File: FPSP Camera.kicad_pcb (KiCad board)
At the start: 4 copper layers, 85.7 x 35 mm, 80 parts, among them J2 Conn_01x02_Pin, J3 USB_B_Micro, J4 SM03B-SRSS-TB, J5 Conn_01x24_Socket, J6 Conn_02x06_Odd_Even, SW1 SW_Push, SW2 SW_Push, U1 RP2350_60QFN, U2 W25Q128JVS, U3 ASM330LHHXTR, U5 TLV74328_SOT23-5, U6 TLV74315_SOT23-5, U7 SiT2001B, U8 NCP1117-3.3_SOT223

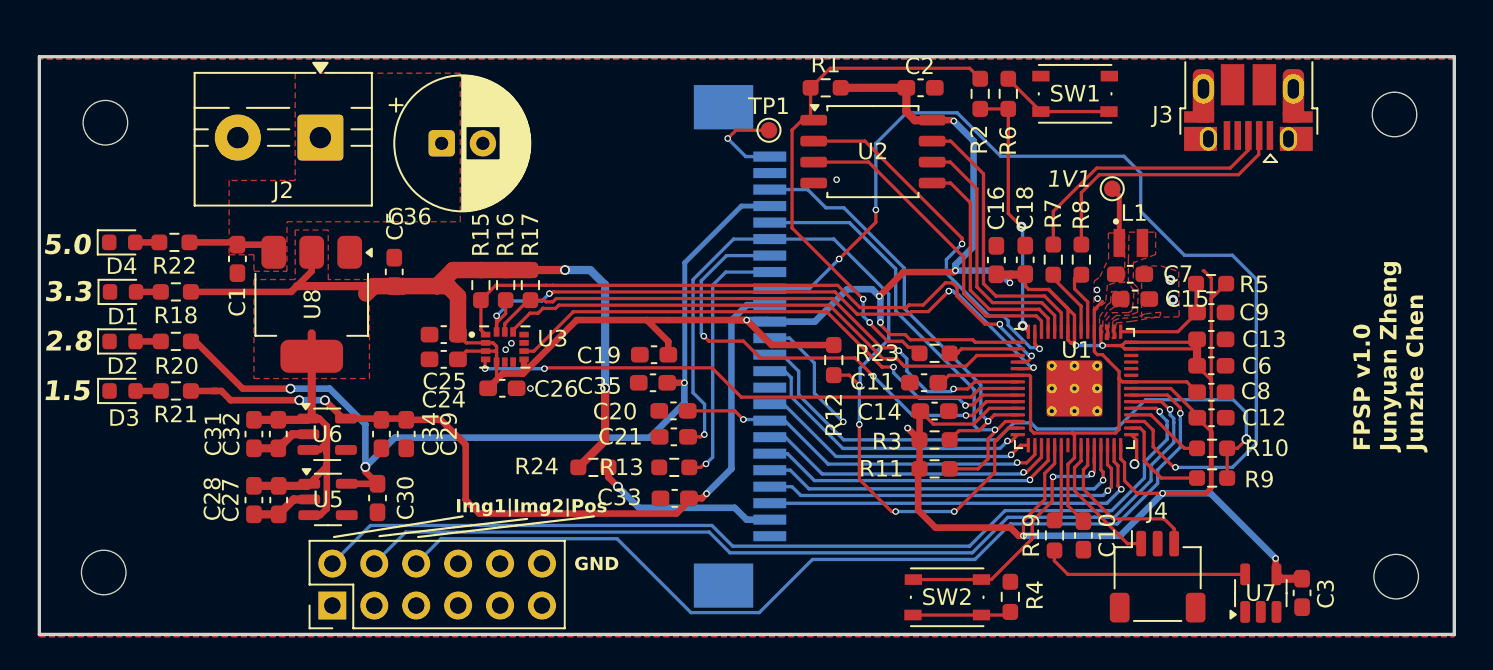
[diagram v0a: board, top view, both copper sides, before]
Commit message: Cleanup
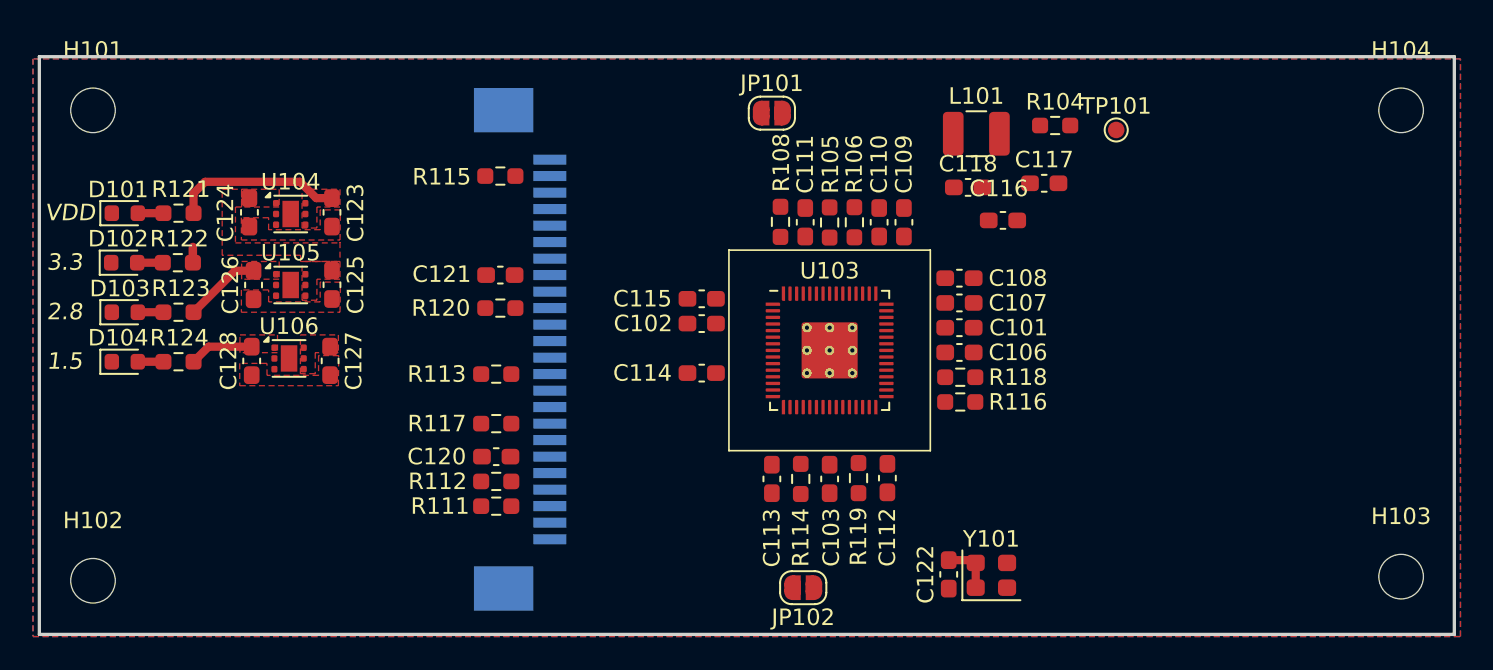
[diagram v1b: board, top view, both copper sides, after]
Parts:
- removed C1, C19, C25, C27, C28, C30, C31, C32, C33, C34, C35, C5: 10u, Capacitor_SMD:C_0603_1608Metric_Pad1.08x0.95mm_HandSolder
- removed C10, C6, C7, C9: 4.7u, Capacitor_SMD:C_0603_1608Metric_Pad1.08x0.95mm_HandSolder
- removed C11, C12, C13, C14, C15, C16, C18, C2, C24, C26, C8: 100n, Capacitor_SMD:C_0603_1608Metric_Pad1.08x0.95mm_HandSolder
- removed C20: 22pF, Capacitor_SMD:C_0603_1608Metric_Pad1.08x0.95mm_HandSolder
- removed C21: 0.1u, Capacitor_SMD:C_0603_1608Metric_Pad1.08x0.95mm_HandSolder
- removed C29: 1u, Capacitor_SMD:C_0603_1608Metric_Pad1.08x0.95mm_HandSolder
- removed C3: 100u, Capacitor_SMD:C_0603_1608Metric_Pad1.08x0.95mm_HandSolder
- removed C36: 10u, Capacitor_THT:CP_Radial_D8.0mm_P2.50mm
- removed D1, D2, D3, D4: LED, Diode_SMD:D_0603_1608Metric
- removed H1, H2, H3, H4: MountingHole, MountingHole:MountingHole_2.7mm_M2.5
- removed J2: Conn_01x02_Pin, TerminalBlock:TerminalBlock_MaiXu_MX126-5.0-02P_1x02_P5.00mm
- removed J3: USB_B_Micro, RP2350_60QFN_minimal:USB_Micro-B_Amphenol_10103594-0001LF_Horizontal_modified
- removed J4: SM03B-SRSS-TB, Connector_JST:JST_SH_SM03B-SRSS-TB_1x03-1MP_P1.00mm_Horizontal
- removed J5: Conn_01x24_Socket, Connector_FFC-FPC:TE_2-84952-4_1x24-1MP_P1.0mm_Horizontal
- removed J6: Conn_02x06_Odd_Even, Connector_PinHeader_2.54mm:PinHeader_2x06_P2.54mm_Vertical
- removed L1: 3.3u, RP2350_60QFN_minimal:L_pol_2016
- removed R1, R19, R23: DNF, Resistor_SMD:R_0603_1608Metric_Pad0.98x0.95mm_HandSolder
- removed R10, R24, R9: 0R, Resistor_SMD:R_0603_1608Metric_Pad0.98x0.95mm_HandSolder
- removed R11, R12, R13, R15, R16, R17, R18, R20, R21, R22, R3: 10k, Resistor_SMD:R_0603_1608Metric_Pad0.98x0.95mm_HandSolder
- removed R2: 0, Resistor_SMD:R_0603_1608Metric_Pad0.98x0.95mm_HandSolder
- removed R4, R6: 1k, Resistor_SMD:R_0603_1608Metric_Pad0.98x0.95mm_HandSolder
- removed R5: 33, Resistor_SMD:R_0603_1608Metric_Pad0.98x0.95mm_HandSolder
- removed R7, R8: 27, Resistor_SMD:R_0603_1608Metric_Pad0.98x0.95mm_HandSolder
- removed SW1, SW2: SW_Push, Button_Switch_SMD:SW_Push_1P1T_NO_Vertical_Wuerth_434133025816
- removed TP1, TP2: TestPoint, TestPoint:TestPoint_Pad_D1.0mm
- removed U1: RP2350_60QFN, RP2350_60QFN_minimal:RP2350-QFN-60-1EP_7x7_P0.4mm_EP3.4x3.4mm_ThermalVias
- removed U2: W25Q128JVS, Package_SO:SOIC-8_5.3x5.3mm_P1.27mm
- removed U3: ASM330LHHXTR, ASM330LHHXTR:XDCR_ASM330LHHXTR
- removed U5: TLV74328_SOT23-5, Package_TO_SOT_SMD:SOT-23-5
- removed U6: TLV74315_SOT23-5, Package_TO_SOT_SMD:SOT-23-5
- removed U7: SiT2001B, Package_TO_SOT_SMD:SOT-23-5
- removed U8: NCP1117-3.3_SOT223, Package_TO_SOT_SMD:SOT-223-3_TabPin2
- added C101: 100n, Capacitor_SMD:C_0603_1608Metric_Pad1.08x0.95mm_HandSolder, F.Cu at (74.8, 28.9)
- added C102: 4.7u, Capacitor_SMD:C_0603_1608Metric_Pad1.08x0.95mm_HandSolder, F.Cu at (59.1, 28.7)
- added C103: 100n, Capacitor_SMD:C_0603_1608Metric_Pad1.08x0.95mm_HandSolder, F.Cu at (66.9, 38.1)
- added C106: 100n, Capacitor_SMD:C_0603_1608Metric_Pad1.08x0.95mm_HandSolder, F.Cu at (74.8, 30.4)
- added C107: 100n, Capacitor_SMD:C_0603_1608Metric_Pad1.08x0.95mm_HandSolder, F.Cu at (74.8, 27.4)
- added C108: 100n, Capacitor_SMD:C_0603_1608Metric_Pad1.08x0.95mm_HandSolder, F.Cu at (74.8, 25.9)
- added C109: 100n, Capacitor_SMD:C_0603_1608Metric_Pad1.08x0.95mm_HandSolder, F.Cu at (71.4, 22.6)
- added C110: 100n, Capacitor_SMD:C_0603_1608Metric_Pad1.08x0.95mm_HandSolder, F.Cu at (69.9, 22.6)
- added C111: 100n, Capacitor_SMD:C_0603_1608Metric_Pad1.08x0.95mm_HandSolder, F.Cu at (65.4, 22.6)
- added C112: 100n, Capacitor_SMD:C_0603_1608Metric_Pad1.08x0.95mm_HandSolder, F.Cu at (70.4, 38.0)
- added C113: 100n, Capacitor_SMD:C_0603_1608Metric_Pad1.08x0.95mm_HandSolder, F.Cu at (63.4, 38.1)
- added C114: 100n, Capacitor_SMD:C_0603_1608Metric_Pad1.08x0.95mm_HandSolder, F.Cu at (59.1, 31.7)
- added C115: 100n, Capacitor_SMD:C_0603_1608Metric_Pad1.08x0.95mm_HandSolder, F.Cu at (59.1, 27.2)
- added C116: 4.7u, Capacitor_SMD:C_0603_1608Metric_Pad1.08x0.95mm_HandSolder, F.Cu at (77.4, 22.4)
- added C117: 4.7u, Capacitor_SMD:C_0603_1608Metric_Pad1.08x0.95mm_HandSolder, F.Cu at (79.9, 20.2)
- added C118: 4.7u, Capacitor_SMD:C_0603_1608Metric_Pad1.08x0.95mm_HandSolder, F.Cu at (75.3, 20.4)
- added C120: 0.1u, Capacitor_SMD:C_0603_1608Metric_Pad1.08x0.95mm_HandSolder, F.Cu at (46.7, 36.8)
- added C121: 22pF, Capacitor_SMD:C_0603_1608Metric_Pad1.08x0.95mm_HandSolder, F.Cu at (47.0, 25.8)
- added C122: 100n, Capacitor_SMD:C_0603_1608Metric_Pad1.08x0.95mm_HandSolder, F.Cu at (74.1, 43.9)
- added C123: 1u, Capacitor_SMD:C_0603_1608Metric_Pad1.08x0.95mm_HandSolder, F.Cu at (36.8, 21.9)
- added C124: 1u, Capacitor_SMD:C_0603_1608Metric_Pad1.08x0.95mm_HandSolder, F.Cu at (31.8, 21.9)
- added C125: 1u, Capacitor_SMD:C_0603_1608Metric_Pad1.08x0.95mm_HandSolder, F.Cu at (36.8, 26.3)
- added C126: 1u, Capacitor_SMD:C_0603_1608Metric_Pad1.08x0.95mm_HandSolder, F.Cu at (32.0, 26.4)
- added C127: 1u, Capacitor_SMD:C_0603_1608Metric_Pad1.08x0.95mm_HandSolder, F.Cu at (36.6, 30.9)
- added C128: 1u, Capacitor_SMD:C_0603_1608Metric_Pad1.08x0.95mm_HandSolder, F.Cu at (31.9, 30.9)
- added D101: LED, Diode_SMD:D_0603_1608Metric, F.Cu at (24.2, 22.0)
- added D102: LED, Diode_SMD:D_0603_1608Metric, F.Cu at (24.2, 25.0)
- added D103: LED, Diode_SMD:D_0603_1608Metric, F.Cu at (24.2, 28.0)
- added D104: LED, Diode_SMD:D_0603_1608Metric, F.Cu at (24.2, 31.0)
- added H101: MountingHole, MountingHole:MountingHole_2.7mm_M2.5, F.Cu at (22.3, 15.8)
- added H102: MountingHole, MountingHole:MountingHole_2.7mm_M2.5, F.Cu at (22.3, 44.3)
- added H103: MountingHole, MountingHole:MountingHole_2.7mm_M2.5, F.Cu at (101.5, 44.0)
- added H104: MountingHole, MountingHole:MountingHole_2.7mm_M2.5, F.Cu at (101.5, 15.8)
- added J101: Conn_01x24_Socket, Connector_FFC-FPC:TE_2-84952-4_1x24-1MP_P1.0mm_Horizontal, B.Cu at (48.1, 30.2)
- added JP101: SolderJumper_2_Open, Jumper:SolderJumper-2_P1.3mm_Open_RoundedPad1.0x1.5mm, F.Cu at (63.4, 15.9)
- added JP102: SolderJumper_2_Open, Jumper:SolderJumper-2_P1.3mm_Open_RoundedPad1.0x1.5mm, F.Cu at (65.3, 44.7)
- added L101: 3.3u, Inductor_SMD:L_1210_3225Metric, F.Cu at (75.8, 17.2)
- added R104: 33, Resistor_SMD:R_0603_1608Metric_Pad0.98x0.95mm_HandSolder, F.Cu at (80.6, 16.7)
- added R105: 27, Resistor_SMD:R_0603_1608Metric_Pad0.98x0.95mm_HandSolder, F.Cu at (66.9, 22.6)
- added R106: 27, Resistor_SMD:R_0603_1608Metric_Pad0.98x0.95mm_HandSolder, F.Cu at (68.4, 22.6)
- added R108: 1k, Resistor_SMD:R_0603_1608Metric_Pad0.98x0.95mm_HandSolder, F.Cu at (63.9, 22.5)
- added R111: 10k, Resistor_SMD:R_0603_1608Metric_Pad0.98x0.95mm_HandSolder, F.Cu at (46.7, 39.8)
- added R112: 10k, Resistor_SMD:R_0603_1608Metric_Pad0.98x0.95mm_HandSolder, F.Cu at (46.7, 38.2)
- added R113: 10k, Resistor_SMD:R_0603_1608Metric_Pad0.98x0.95mm_HandSolder, F.Cu at (46.7, 31.8)
- added R114: DNF, Resistor_SMD:R_0603_1608Metric_Pad0.98x0.95mm_HandSolder, F.Cu at (65.2, 38.1)
- added R115: 0R, Resistor_SMD:R_0603_1608Metric_Pad0.98x0.95mm_HandSolder, F.Cu at (47.0, 19.8)
- added R116: 0R, Resistor_SMD:R_0603_1608Metric_Pad0.98x0.95mm_HandSolder, F.Cu at (74.8, 33.4)
- added R117: 10k, Resistor_SMD:R_0603_1608Metric_Pad0.98x0.95mm_HandSolder, F.Cu at (46.7, 34.8)
- added R118: 0R, Resistor_SMD:R_0603_1608Metric_Pad0.98x0.95mm_HandSolder, F.Cu at (74.8, 31.9)
- added R119: 1k, Resistor_SMD:R_0603_1608Metric_Pad0.98x0.95mm_HandSolder, F.Cu at (68.7, 38.0)
- added R120: 0R, Resistor_SMD:R_0603_1608Metric_Pad0.98x0.95mm_HandSolder, F.Cu at (47.0, 27.8)
- added R121: 10k, Resistor_SMD:R_0603_1608Metric_Pad0.98x0.95mm_HandSolder, F.Cu at (27.4, 22.0)
- added R122: 10k, Resistor_SMD:R_0603_1608Metric_Pad0.98x0.95mm_HandSolder, F.Cu at (27.4, 25.0)
- added R123: 10k, Resistor_SMD:R_0603_1608Metric_Pad0.98x0.95mm_HandSolder, F.Cu at (27.4, 28.0)
- added R124: 10k, Resistor_SMD:R_0603_1608Metric_Pad0.98x0.95mm_HandSolder, F.Cu at (27.4, 31.0)
- added TP101: TestPoint, TestPoint:TestPoint_Pad_D1.0mm, F.Cu at (84.3, 17.0)
- added U103: RP2350_60QFN, projLib:RP2350-QFN-60-1EP_7x7_P0.4mm_EP3.4x3.4mm_ThermalVias, F.Cu at (66.9, 30.3)
- added U104: TLV75533PDRV, Package_SON:WSON-6-1EP_2x2mm_P0.65mm_EP1x1.6mm, F.Cu at (34.2, 22.1)
- added U105: TLV73328PDRV, Package_SON:WSON-6-1EP_2x2mm_P0.65mm_EP1x1.6mm, F.Cu at (34.2, 26.4)
- added U106: TLV73315PDRV, Package_SON:WSON-6-1EP_2x2mm_P0.65mm_EP1x1.6mm, F.Cu at (34.1, 30.8)
- added Y101: SiT8008xx-1x-xxE, Oscillator:Oscillator_SMD_SiT_PQFN-4Pin_2.5x2.0mm, F.Cu at (76.7, 43.9)
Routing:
- net +3.3V: track 263.2 -> 5.07 mm, vias 14 -> 0
- net HSYNC_1: track 62.0 -> 0.00 mm, vias 3 -> 0
- net POSITION_OUT_1: track 59.1 -> 0.00 mm, vias 1 -> 0
- net IMAGE_OUT_1_1: track 59.0 -> 0.00 mm, vias 1 -> 0
- net IMAGE_OUT_2_1: track 57.7 -> 0.00 mm, vias 1 -> 0
- net ~{RESET_1}: track 52.3 -> 0.00 mm, vias 5 -> 0
- net +2V8: track 56.5 -> 4.68 mm, vias 3 -> 0
- net +1V5: track 50.8 -> 3.90 mm, vias 3 -> 0
- net SDO_imu_1: track 40.4 -> 0.00 mm, vias 2 -> 0
- net SDA_imu_1: track 40.2 -> 0.00 mm, vias 4 -> 0
- net /IOs/XCLK: track 38.3 -> 0.00 mm, vias 1 -> 0
- net +1V1: track 37.8 -> 0.00 mm, vias 2 -> 0
- net SCL_imu_1: track 35.3 -> 0.00 mm, vias 2 -> 0
- net INT1_1: track 33.8 -> 0.00 mm, vias 2 -> 0
- net INT2_1: track 33.7 -> 0.00 mm, vias 2 -> 0
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- added copper zone on B.Cu, net (none)
- added copper zone on F.Cu, net (none)
- added copper zone on F.Cu, net +1V5
- added copper zone on F.Cu, net +2V8
- added copper zone on F.Cu, net AGND
- removed copper zone on F.Cu, net +1V1
- removed copper zone on F.Cu, net /MCU/VREG_LX_1
- removed copper zone on B.Cu, net GND
- removed copper zone on F.Cu, net GND
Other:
- board text added: "VDD"
- board text removed: "1V1"
- board text removed: "5.0"
- board text removed: "FPSP v1.0 Junyuan Zheng Junzhe Chen"
- board text removed: "GND"
- board text removed: "Img1|Img2|Pos"
